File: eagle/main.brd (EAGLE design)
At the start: 55 x 127 mm, 108 parts, among them IC1 LD117AS50TR, IC2 LD117AS33TR, IC3 OPA340U, Q1 BSS138, Q2 BSS138, T1 FDV304P, U1 STM32F777VIT, U2 CG2179M2, U3 L272, U4 ADAM TECH MCSP-Q1-08-A-SG, U5 SI4463-C2A-GM, X1 16MHz, X2 SMA, X3 ILSI 32MHz TCXO

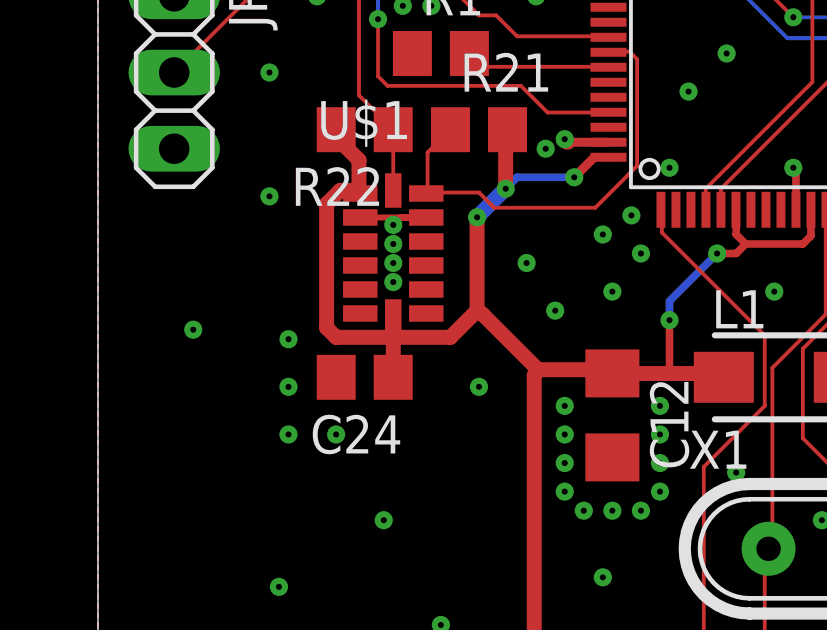
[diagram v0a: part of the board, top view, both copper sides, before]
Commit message: Add files via upload
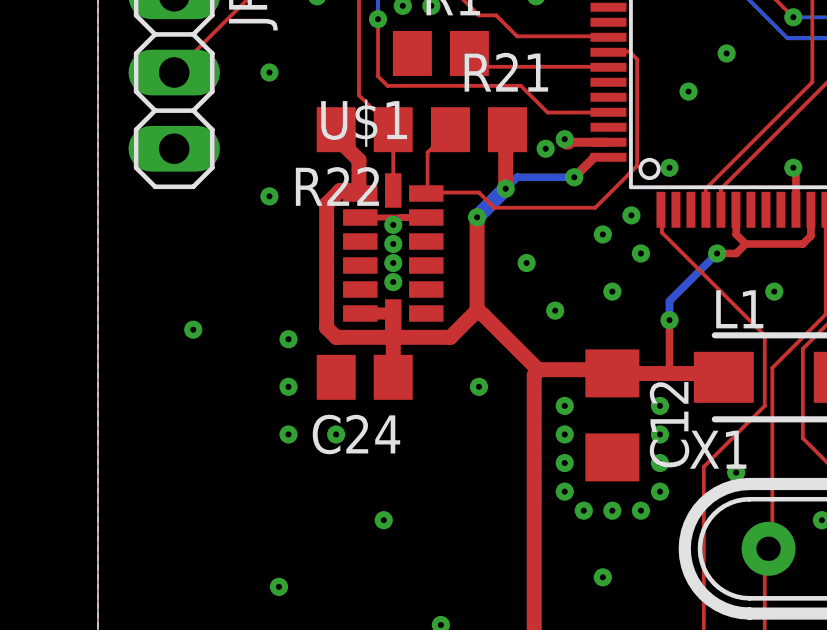
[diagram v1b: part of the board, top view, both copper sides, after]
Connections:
- net +3V3: now also U$1.P$6
- net GND: no longer U$1.P$6
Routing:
- net +3V3: track 367.5 -> 368.7 mm
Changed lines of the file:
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@@
 </class>
 </classes>
-<designrules name="Moje Technoservice 2">
+<designrules name="Moje Technoservice 2 *">
 <description language="de">&lt;b&gt;EAGLE Design Rules&lt;/b&gt;
 &lt;p&gt;
@@
 <param name="mlMinCreamFrame" value="0mil"/>
 <param name="mlMaxCreamFrame" value="0mil"/>
-<param name="mlViaStopLimit" value="0mil"/>
+<param name="mlViaStopLimit" value="0.3mm"/>
 <param name="srRoundness" value="0"/>
 <param name="srMinRoundness" value="0mil"/>
@@
 <contactref element="Q2" pad="2"/>
 <contactref element="U3" pad="6"/>
-<contactref element="U$1" pad="P$6"/>
 <contactref element="U$1" pad="P$5"/>
 <contactref element="U$1" pad="P$4"/>
@@
 <wire x1="40.3225" y1="93.98" x2="40.3225" y2="95.6945" width="0.3" layer="1"/>
 <wire x1="40.3225" y1="95.6945" x2="40.1955" y2="95.8215" width="0.3" layer="1"/>
+<contactref element="U$1" pad="P$6"/>
+<wire x1="8.7425" y1="37.0525" x2="9.8425" y2="37.0525" width="0.4064" layer="1"/>
+<wire x1="9.8425" y1="37.0525" x2="9.8425" y2="36.9525" width="0.4064" layer="1"/>
 </signal>
 <signal name="SWDIO">
